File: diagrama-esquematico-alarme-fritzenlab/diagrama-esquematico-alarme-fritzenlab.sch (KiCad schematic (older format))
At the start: 20 parts, among them J1 ESP-12 WiFi, J2 Sirene, J3 Sensores, J4 Teclado, J5 Display_LCD, J6a1 Conn_01x04_Female, J6b1 Conn_01x04_Female, J7 Antena_Radio, Q1 TIP120, U1 DHT11

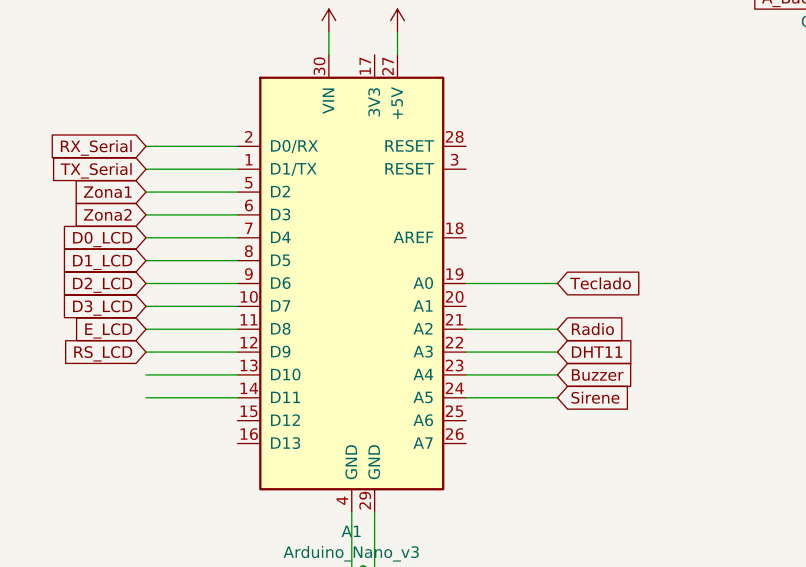
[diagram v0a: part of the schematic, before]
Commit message: modificado esquematico e codigo
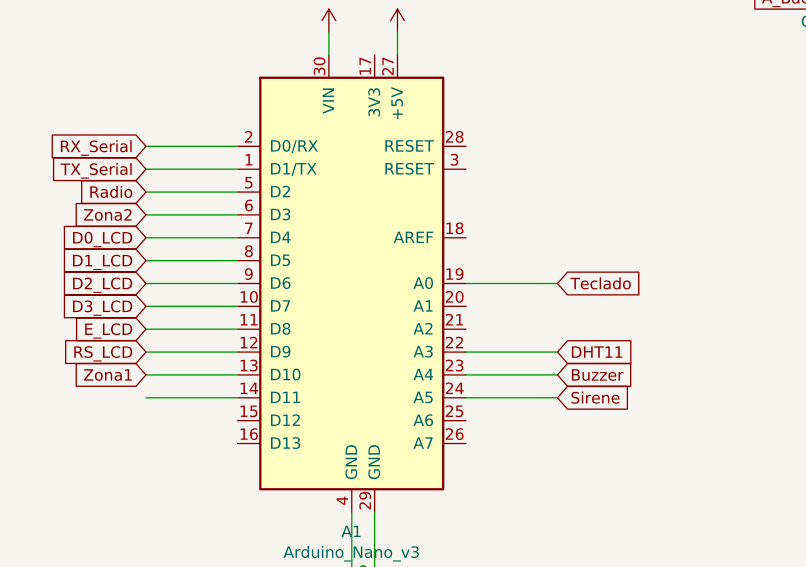
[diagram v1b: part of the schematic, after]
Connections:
- net Radio: now also A1.5 (D2); no longer A1.21 (A2)
- net Zona1: now also A1.13 (D10); no longer A1.5 (D2)
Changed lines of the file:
@@
 Wire Wire Line
 	4900 3950 4500 3950
-Text GLabel 4500 3050 0    50   Input ~ 0
+Text GLabel 4500 3850 0    50   Input ~ 0
 Zona1
 Text GLabel 4500 3150 0    50   Input ~ 0
@@
 Text GLabel 4500 3550 0    50   Input ~ 0
 D3_LCD
-Wire Wire Line
-	5900 3650 6300 3650
-Text GLabel 6300 3650 2    50   Input ~ 0
+Text GLabel 4500 3050 0    50   Input ~ 0
 Radio
 $Comp
